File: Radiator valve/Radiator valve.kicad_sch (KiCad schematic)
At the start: 48 parts, among them J1 53047-0410, J2 USB4105-GF-A-120, J4 Conn_01x03, M1 Stepper_Motor, U1 MLX90632SLD-BCB-000-SP, U2 ESP32-S3-MINI-1, U3 TPS63031DSK, U4 BQ24075RGT, U6 DRV8833PW

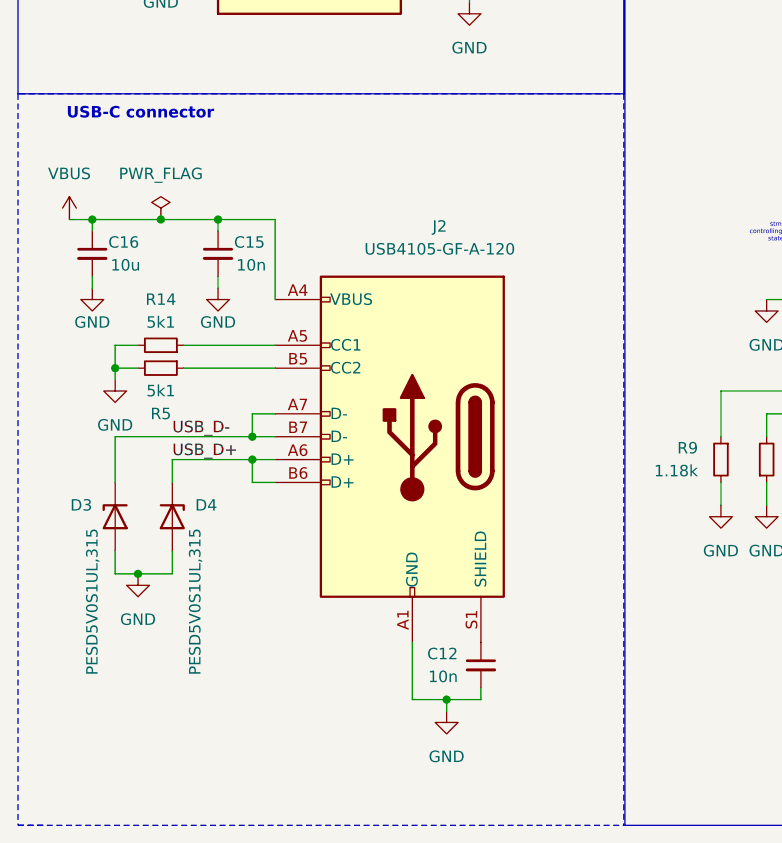
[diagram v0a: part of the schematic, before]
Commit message: FInal
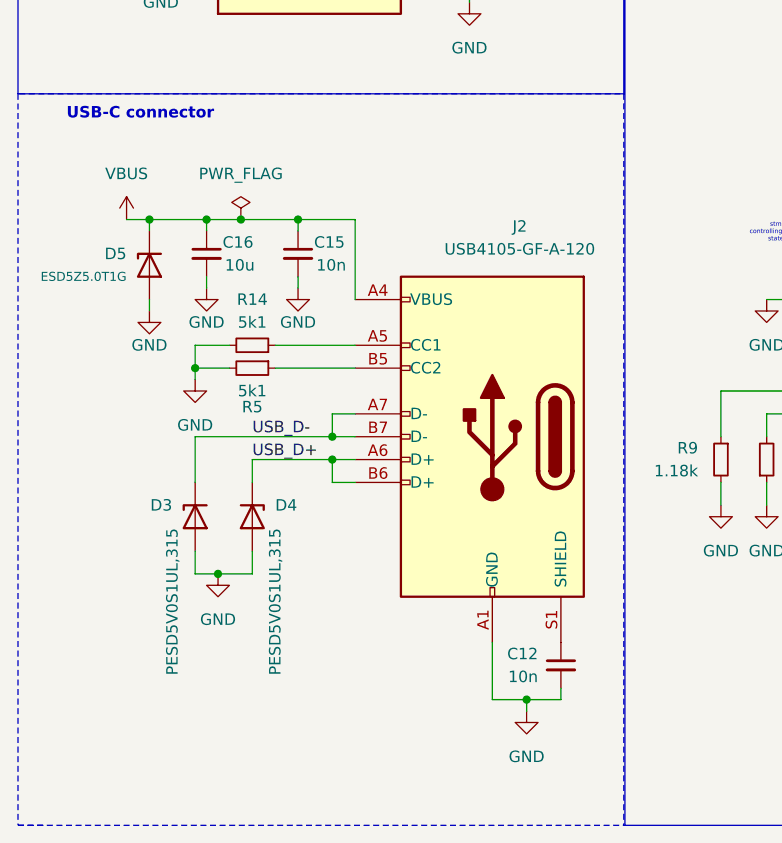
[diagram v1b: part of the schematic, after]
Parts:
- added D5: ESD5Z5.0T1G, Diode_SMD:D_SOD-523, symbol Diode:ESD5Zxx
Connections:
- net GND: now also D5.2 (A)
- net VBUS: now also D5.1 (K)
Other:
- moved on the sheet: C12, C15, C16, D3, D4, J2, R14, R5
